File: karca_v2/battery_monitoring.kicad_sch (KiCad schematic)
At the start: 15 parts, among them U33 INA180A2, U34 MCP3204, U35 NUP4202, U36 TLV9301xDBV

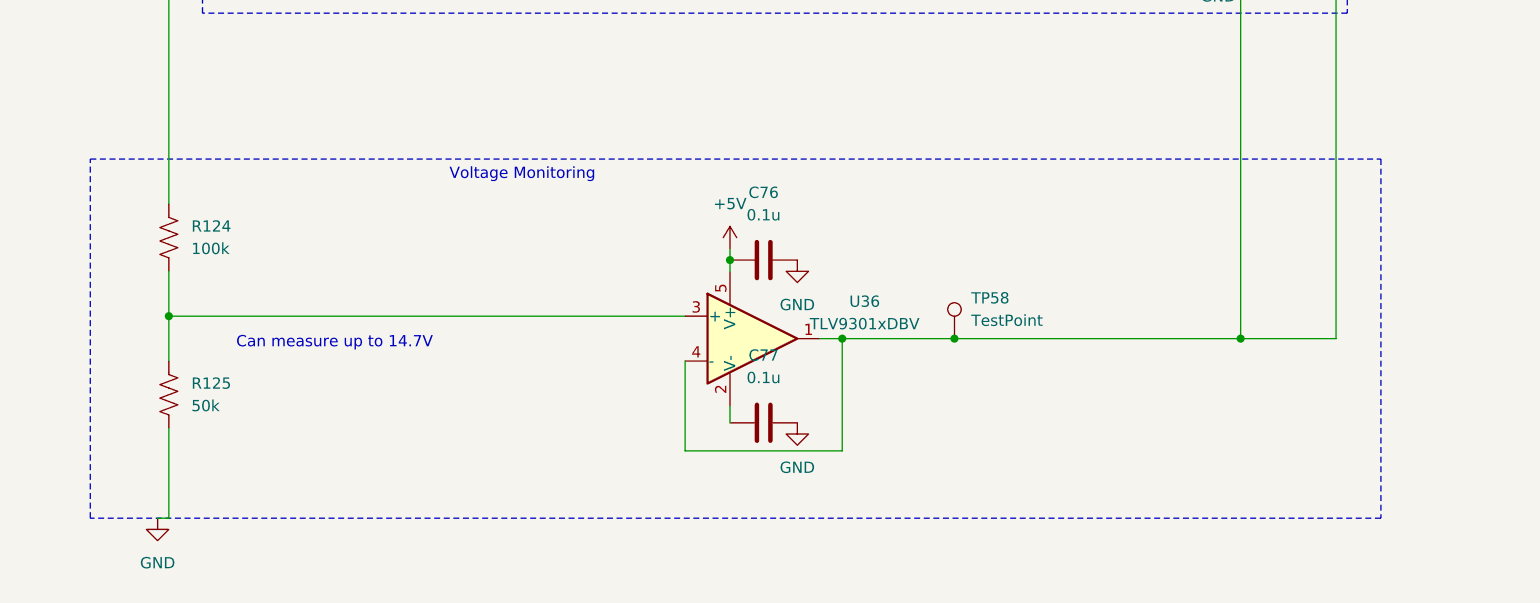
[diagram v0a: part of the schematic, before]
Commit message: revisions for V2.1
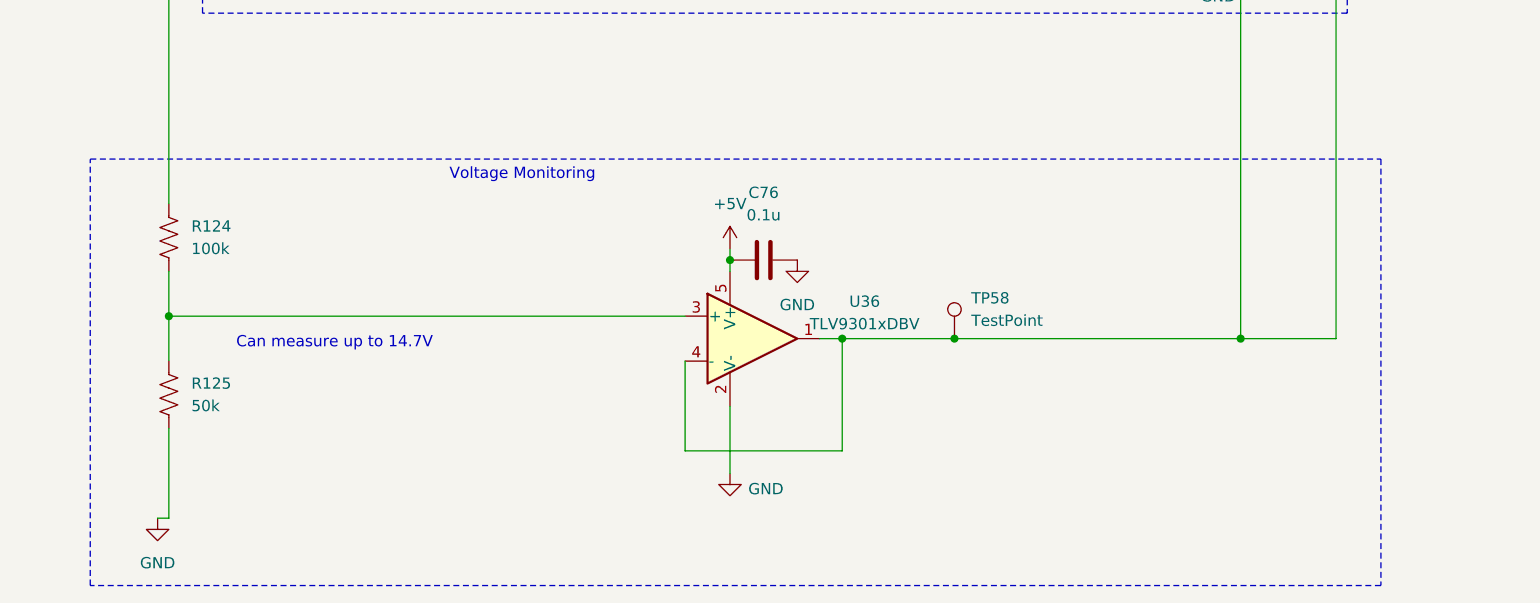
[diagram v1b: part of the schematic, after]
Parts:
- removed C77: 0.1u, Capacitor_SMD:C_0402_1005Metric, symbol Device:C
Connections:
- net GND: now also U36.2 (V-)
